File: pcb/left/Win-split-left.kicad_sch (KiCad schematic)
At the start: 158 parts, among them J1 Conn_01x04_Socket, Q1 Q_PMOS_GSD, SW8 ROT_SKYLOONG_HS, U1 RP2040_ProMicro, U3 74AHCT1G125

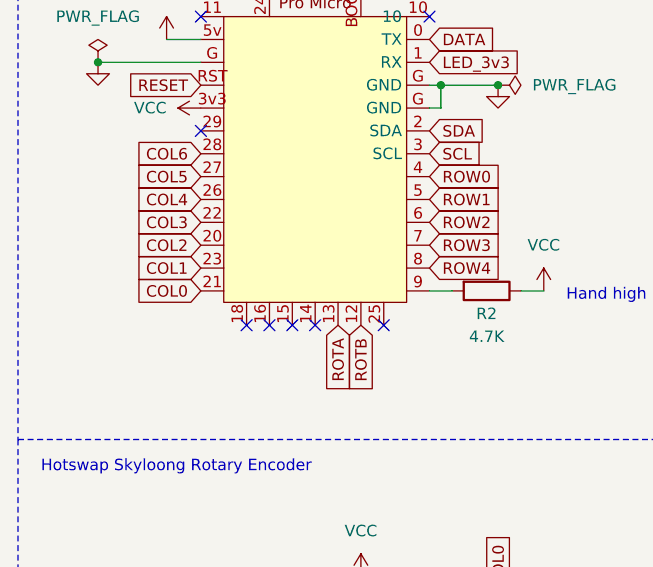
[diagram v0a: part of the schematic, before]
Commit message: designed
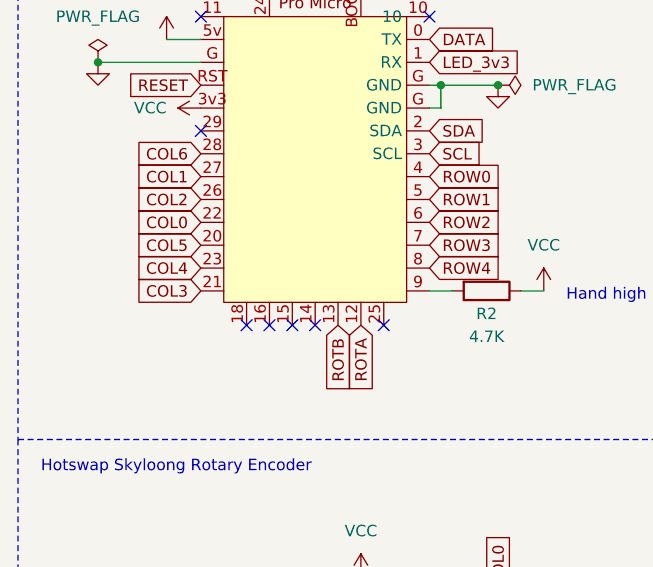
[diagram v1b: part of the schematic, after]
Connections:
- net COL0: now also U1.22; no longer U1.21
- net COL1: now also U1.27; no longer U1.23
- net COL2: now also U1.26; no longer U1.20
- net COL3: now also U1.21; no longer U1.22
- net COL4: now also U1.23; no longer U1.26
- net COL5: now also U1.20; no longer U1.27
- net ROTA: now also U1.12; no longer U1.13
- net ROTB: now also U1.13; no longer U1.12
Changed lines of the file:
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@@
     )
   )
-  (global_label "ROTB" (shape input) (at 53.34 71.12 270) (fields_autoplaced)
+  (global_label "ROTA" (shape input) (at 53.34 71.12 270) (fields_autoplaced)
     (effects (font (size 1.27 1.27)) (justify right))
-    (property "Intersheetrefs" "${INTERSHEET_REFS}" (at 53.34 78.9433 90)
+    (property "Intersheetrefs" "${INTERSHEET_REFS}" (at 53.34 78.7619 90)
       (effects (font (size 1.27 1.27)) (justify right) hide)
     )
@@
     )
   )
-  (global_label "ROTA" (shape input) (at 50.8 71.12 270) (fields_autoplaced)
+  (global_label "ROTB" (shape input) (at 50.8 71.12 270) (fields_autoplaced)
     (effects (font (size 1.27 1.27)) (justify right))
-    (property "Intersheetrefs" "${INTERSHEET_REFS}" (at 50.8 78.7619 90)
+    (property "Intersheetrefs" "${INTERSHEET_REFS}" (at 50.8 78.9433 90)
       (effects (font (size 1.27 1.27)) (justify right) hide)
     )
@@
     )
   )
-  (global_label "COL2" (shape input) (at 35.56 62.23 180) (fields_autoplaced)
+  (global_label "COL5" (shape input) (at 35.56 62.23 180) (fields_autoplaced)
     (effects (font (size 1.27 1.27)) (justify right))
     (property "Intersheetrefs" "${INTERSHEET_REFS}" (at 27.7367 62.23 0)
@@
     )
   )
-  (global_label "COL0" (shape input) (at 35.56 67.31 180) (fields_autoplaced)
+  (global_label "COL3" (shape input) (at 35.56 67.31 180) (fields_autoplaced)
     (effects (font (size 1.27 1.27)) (justify right))
     (property "Intersheetrefs" "${INTERSHEET_REFS}" (at 27.7367 67.31 0)
@@
     )
   )
-  (global_label "COL5" (shape input) (at 35.56 54.61 180) (fields_autoplaced)
+  (global_label "COL1" (shape input) (at 35.56 54.61 180) (fields_autoplaced)
     (effects (font (size 1.27 1.27)) (justify right))
     (property "Intersheetrefs" "${INTERSHEET_REFS}" (at 27.7367 54.61 0)
@@
     )
   )
-  (global_label "COL1" (shape input) (at 35.56 64.77 180) (fields_autoplaced)
+  (global_label "COL4" (shape input) (at 35.56 64.77 180) (fields_autoplaced)
     (effects (font (size 1.27 1.27)) (justify right))
     (property "Intersheetrefs" "${INTERSHEET_REFS}" (at 27.7367 64.77 0)
@@
     )
   )
-  (global_label "COL3" (shape input) (at 35.56 59.69 180) (fields_autoplaced)
+  (global_label "COL0" (shape input) (at 35.56 59.69 180) (fields_autoplaced)
     (effects (font (size 1.27 1.27)) (justify right))
     (property "Intersheetrefs" "${INTERSHEET_REFS}" (at 27.7367 59.69 0)
@@
     )
   )
-  (global_label "COL4" (shape input) (at 35.56 57.15 180) (fields_autoplaced)
+  (global_label "COL2" (shape input) (at 35.56 57.15 180) (fields_autoplaced)
     (effects (font (size 1.27 1.27)) (justify right))
     (property "Intersheetrefs" "${INTERSHEET_REFS}" (at 27.7367 57.15 0)
